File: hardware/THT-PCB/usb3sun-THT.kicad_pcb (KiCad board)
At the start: 2 copper layers, 91 x 48.3 mm, 46 parts, among them J2 8918-P8B, J3 USB-U267-BWS, Q1 2N7000, Q2 2N7000, Q3 2N7000, Q4 2N7000, Q5 2N7000, Q6 2N7000, SW1 TS665CJ, U1 Pico, U2 SRV05-4, U4 MAX40200AUK, U5 MAX40200AUK

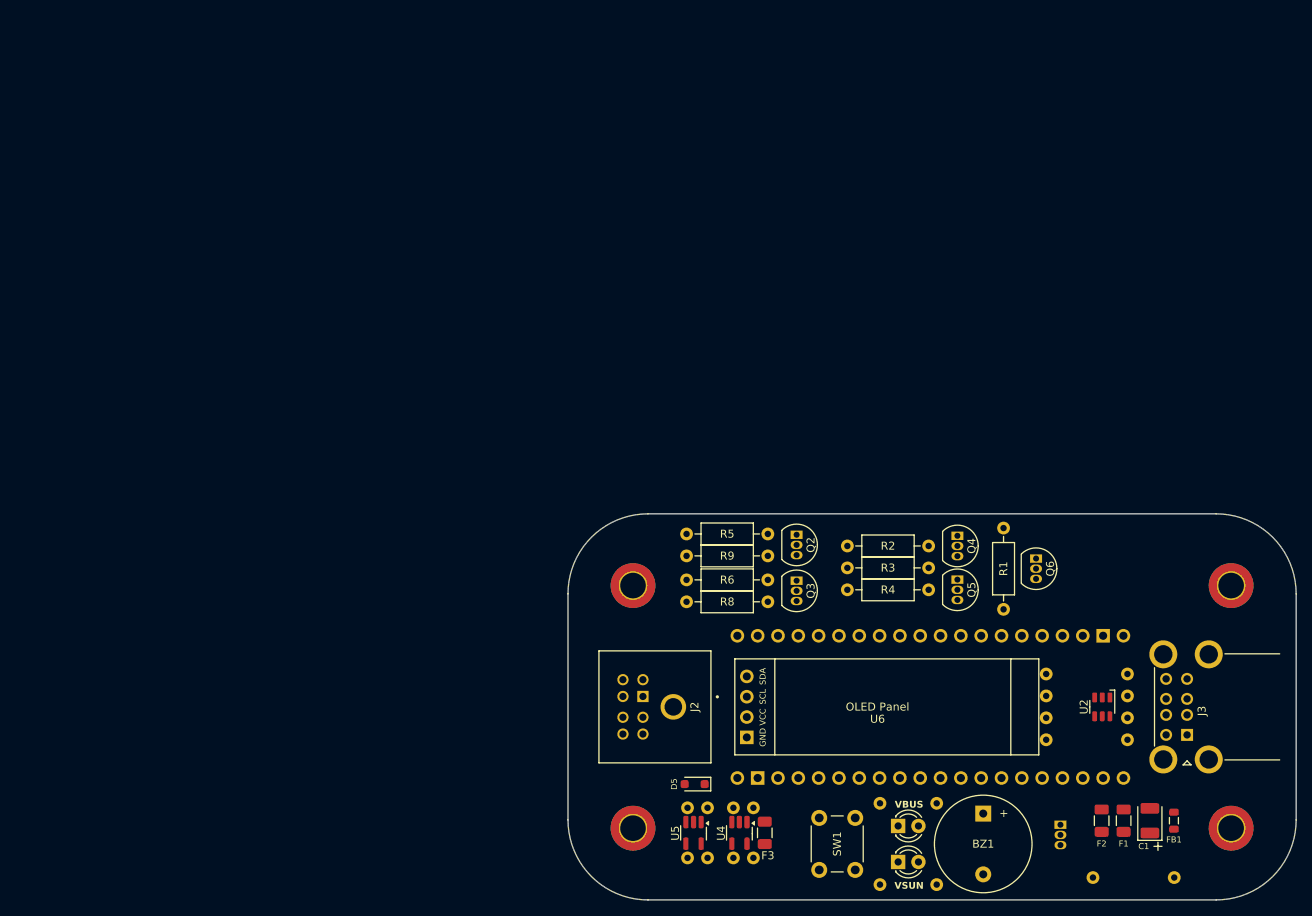
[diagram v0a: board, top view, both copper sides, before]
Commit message: Fully Routed
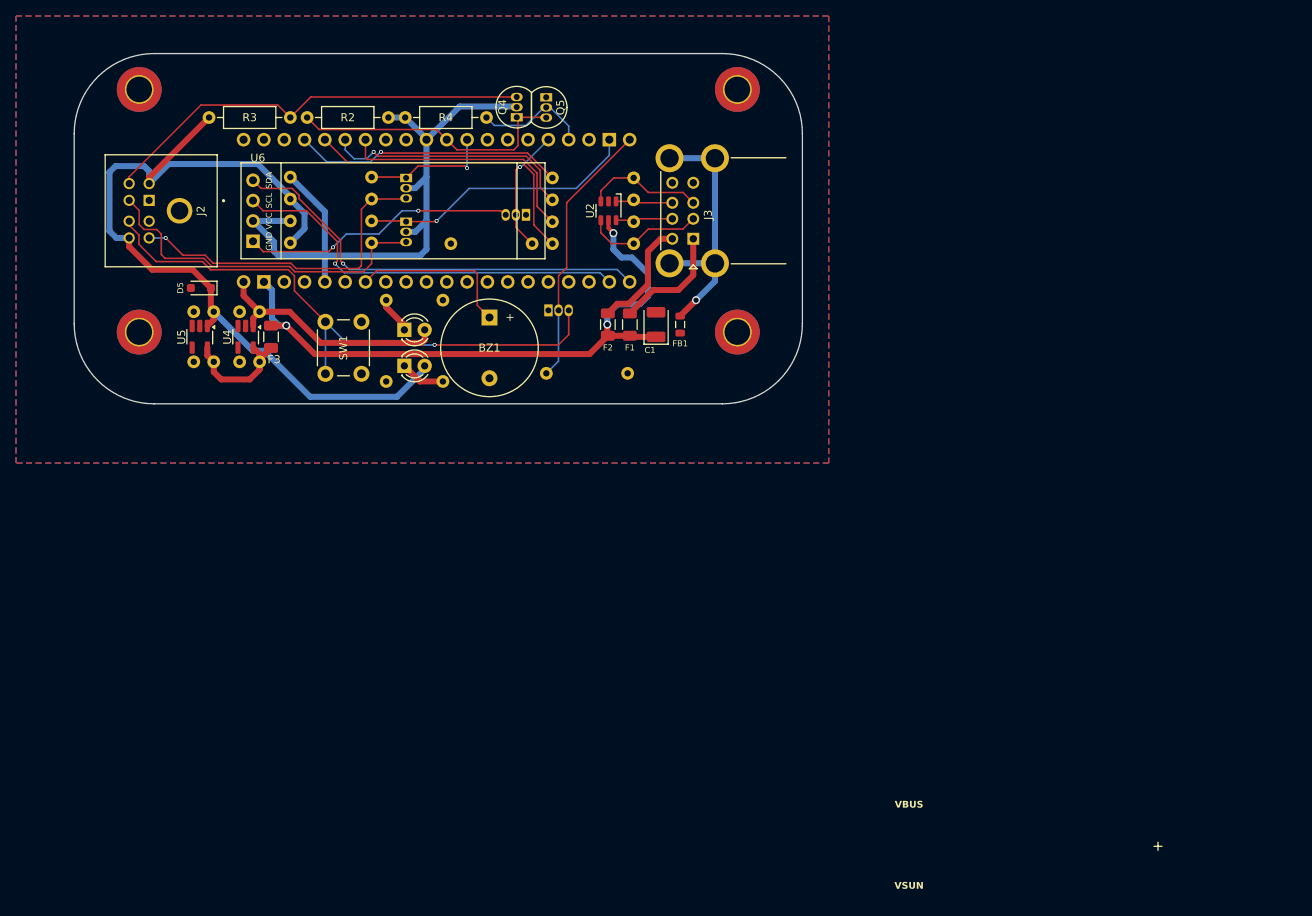
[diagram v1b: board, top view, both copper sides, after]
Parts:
- Q2, Q3, Q6, R1, R5, R6, R8, R9: moved to B.Cu
- moved R3 97.7 mm to (74.9, 48.2)
- moved R7 93.0 mm to (117.1, 80.2)
- moved Q1 90.7 mm to (117.3, 72.4), turned to 0 degrees
- moved R14 88.1 mm to (104.2, 81.2)
- moved R15 88.1 mm to (97.1, 71.1)
- moved C1 87.5 mm to (130.8, 74.1)
- moved D1 87.5 mm to (99.3, 74.8)
- moved D4 87.5 mm to (99.3, 79.3)
- moved H2 87.5 mm to (141.0, 75.1)
- moved H3 87.5 mm to (66.2, 44.7)
- moved H4 87.5 mm to (66.2, 75.1)
- moved J2 87.5 mm to (75.9, 59.9)
- moved U6 87.5 mm to (116.9, 65.9)
- moved D5 87.5 mm to (73.9, 69.6)
- moved F1 87.5 mm to (127.5, 74.1)
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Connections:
- R10 pad 1: /D2+ -> /D1+
- R10 pad 2: /INT_D2+ -> /INT_D1+
- R11 pad 1: /D2- -> /D2+
- R11 pad 2: /INT_D2- -> /INT_D2+
- R12 pad 1: /D1+ -> /D1-
- R12 pad 2: /INT_D1+ -> /INT_D1-
- R13 pad 1: /D1- -> /D2-
- R13 pad 2: /INT_D1- -> /INT_D2-
- U2 pad 1: /D2+ -> /D1+
- U2 pad 3: /D2- -> /D2+
- U2 pad 4: /D1- -> /D2-
- U2 pad 6: /D1+ -> /D1-
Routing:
- net VSUN: track 0.00 -> 107.5 mm
- net +3V3: track 0.00 -> 88.8 mm
- net +5V: track 0.00 -> 78.8 mm, vias 0 -> 3
- net /SPOWER: track 0.00 -> 73.5 mm, vias 0 -> 1
- net /KTX: track 0.00 -> 54.7 mm
- net /DISPLAY_SDA: track 0.00 -> 54.1 mm, vias 0 -> 1
- net /DISPLAY_SCL: track 0.00 -> 50.8 mm, vias 0 -> 1
- net /MTX: track 0.00 -> 43.9 mm
- net /KRX: track 0.00 -> 41.5 mm, vias 0 -> 1
- net /INT_D2-: track 0.00 -> 37.5 mm
- net /INT_KTX: track 0.00 -> 35.6 mm
- net /INT_MTX: track 0.00 -> 35.1 mm, vias 0 -> 1
- net /DISPLAY_GND: track 0.00 -> 34.5 mm, vias 0 -> 2
- net /INT_D2+: track 0.00 -> 34.0 mm, vias 0 -> 1
- net /INT_SPOWER: track 0.00 -> 33.5 mm
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- added copper zone on B.Cu, net GND
- added copper zone on F.Cu, net GND
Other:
- board size 91 x 48.3 mm -> 91 x 43.8 mm
